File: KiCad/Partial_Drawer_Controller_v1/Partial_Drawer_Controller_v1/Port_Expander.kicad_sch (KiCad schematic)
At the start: 3 parts, among them U5 PCA9554PW,118

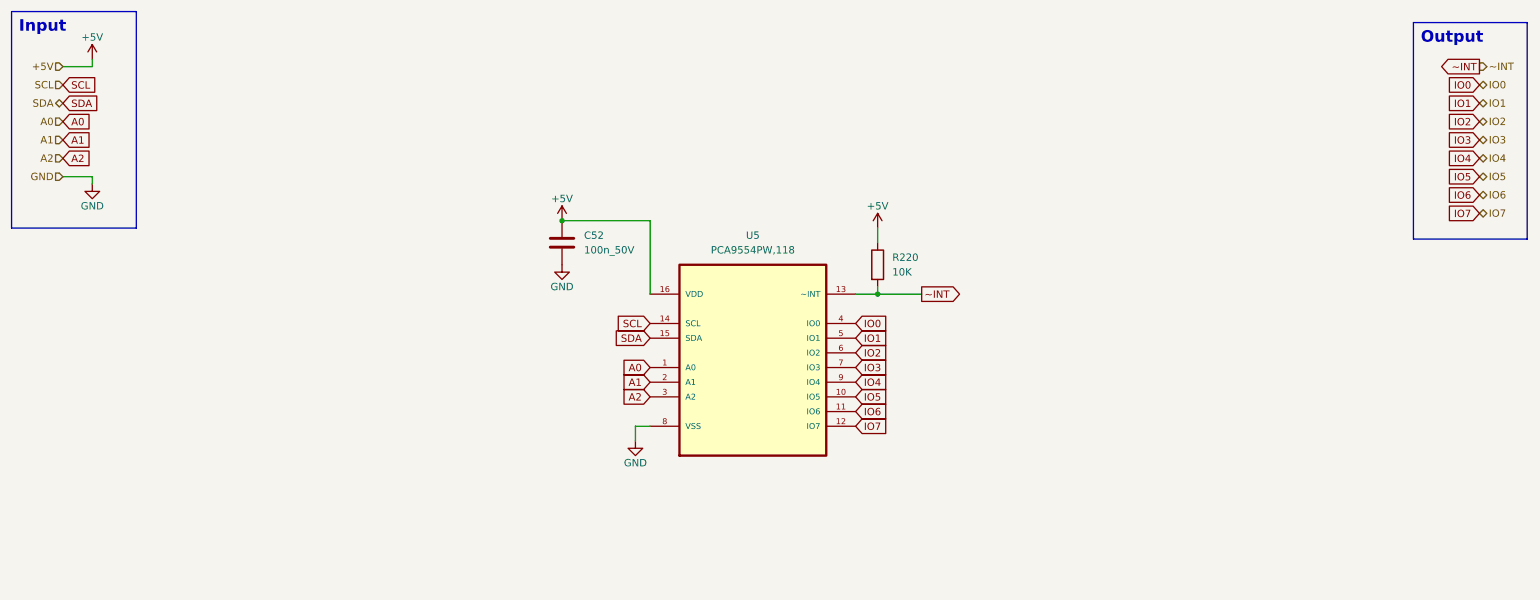
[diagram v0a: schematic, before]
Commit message: feat: finishing first draft for `partial_drawer_controller_v1` schematic
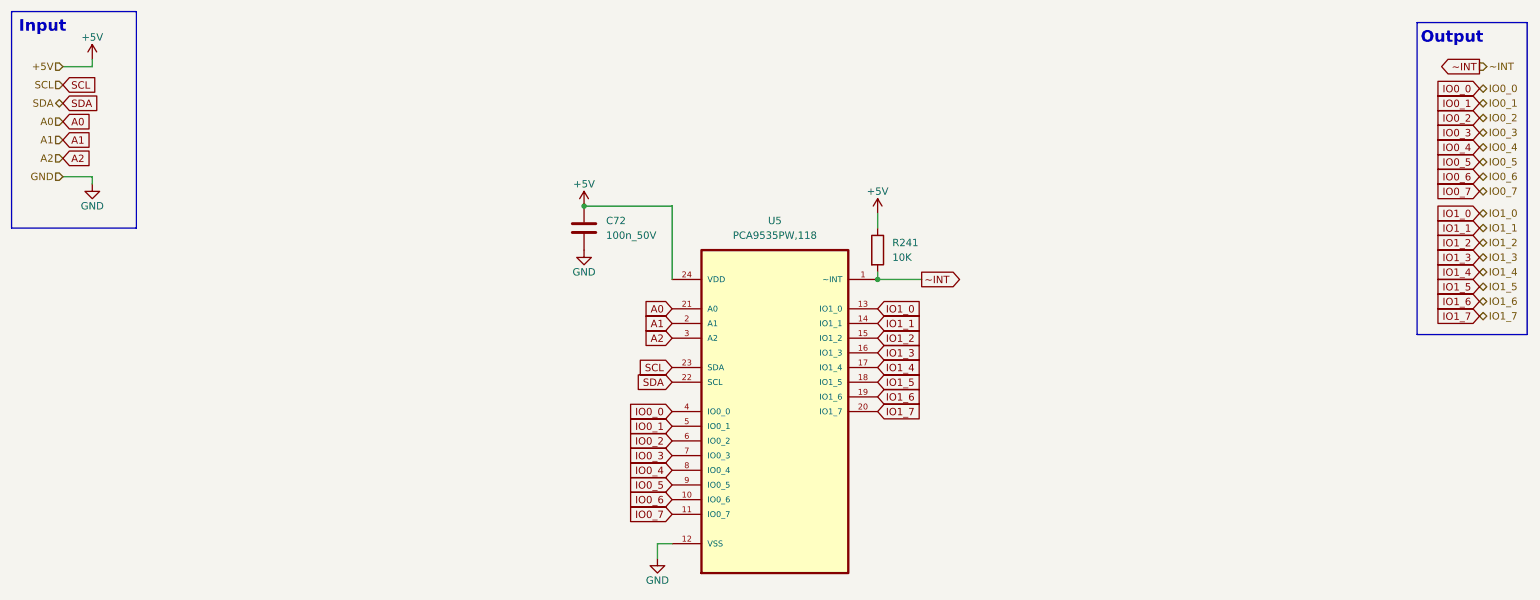
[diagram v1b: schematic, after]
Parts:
- removed C52: 100n_50V, Capacitor_SMD:C_0402_1005Metric, symbol _C_0402:100n_50V
- removed R220: 10K, Resistor_SMD:R_0402_1005Metric, symbol _R_0402:10K
- removed U5: PCA9554PW,118, Package_SO:TSSOP-16_4.4x5mm_P0.65mm, symbol _Interface_Expansion:PCA9554PW,118
- added C72: 100n_50V, Capacitor_SMD:C_0402_1005Metric, symbol _C_0402:100n_50V
- added R241: 10K, Resistor_SMD:R_0402_1005Metric, symbol _R_0402:10K
- added U5: PCA9535PW,118, Package_SO:TSSOP-24_4.4x7.8mm_P0.65mm, symbol _Interface_Expansion:PCA9535PW,118
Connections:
- net +5V: now also C72.1, R241.1, U5.24 (VDD)
- net A0: now also U5.21 (A0)
- net A1: now also U5.2 (A1)
- net A2: now also U5.3 (A2)
- net GND: now also C72.2, U5.12 (VSS)
- net SCL: now also U5.23 (SDA)
- net SDA: now also U5.22 (SCL)
- net ~INT: now also R241.2, U5.1 (~INT)
- new net IO0_0: U5.4 (IO0_0)
- new net IO0_1: U5.5 (IO0_1)
- new net IO0_2: U5.6 (IO0_2)
- new net IO0_3: U5.7 (IO0_3)
- new net IO0_4: U5.8 (IO0_4)
- new net IO0_5: U5.9 (IO0_5)
- new net IO0_6: U5.10 (IO0_6)
- new net IO0_7: U5.11 (IO0_7)
- new net IO1_0: U5.13 (IO1_0)
- new net IO1_1: U5.14 (IO1_1)
- new net IO1_2: U5.15 (IO1_2)
- new net IO1_3: U5.16 (IO1_3)
- new net IO1_4: U5.17 (IO1_4)
- new net IO1_5: U5.18 (IO1_5)
- new net IO1_6: U5.19 (IO1_6)
- new net IO1_7: U5.20 (IO1_7)
